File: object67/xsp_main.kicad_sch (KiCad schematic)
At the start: 67 parts, among them IC5 TPS7A4701RGWT, IC6 TPS7A3301RGWR, J2 PJ-037A, J3 Power In, J4 216700-0249, U10 ADP5070AREZ, U11 TPS62912, U7 TPS7A2050PDQNR, U8 TPS7A2033PDQNR, U9 TPS7A2033PDQNR

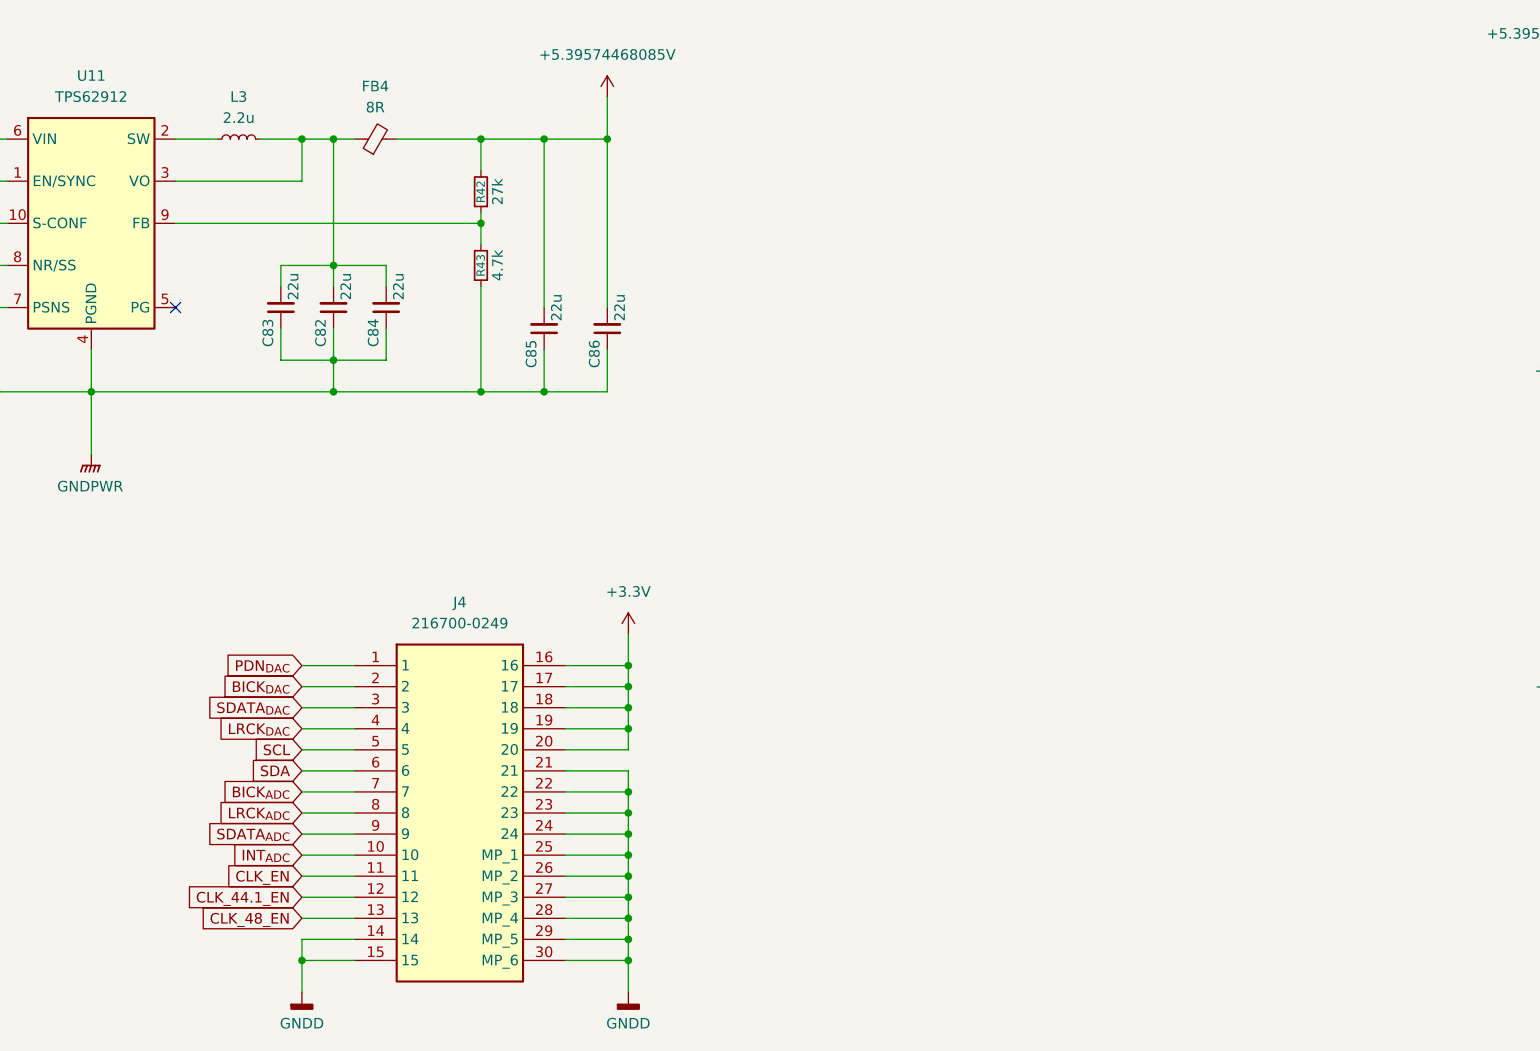
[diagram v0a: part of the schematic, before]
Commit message: Start layout
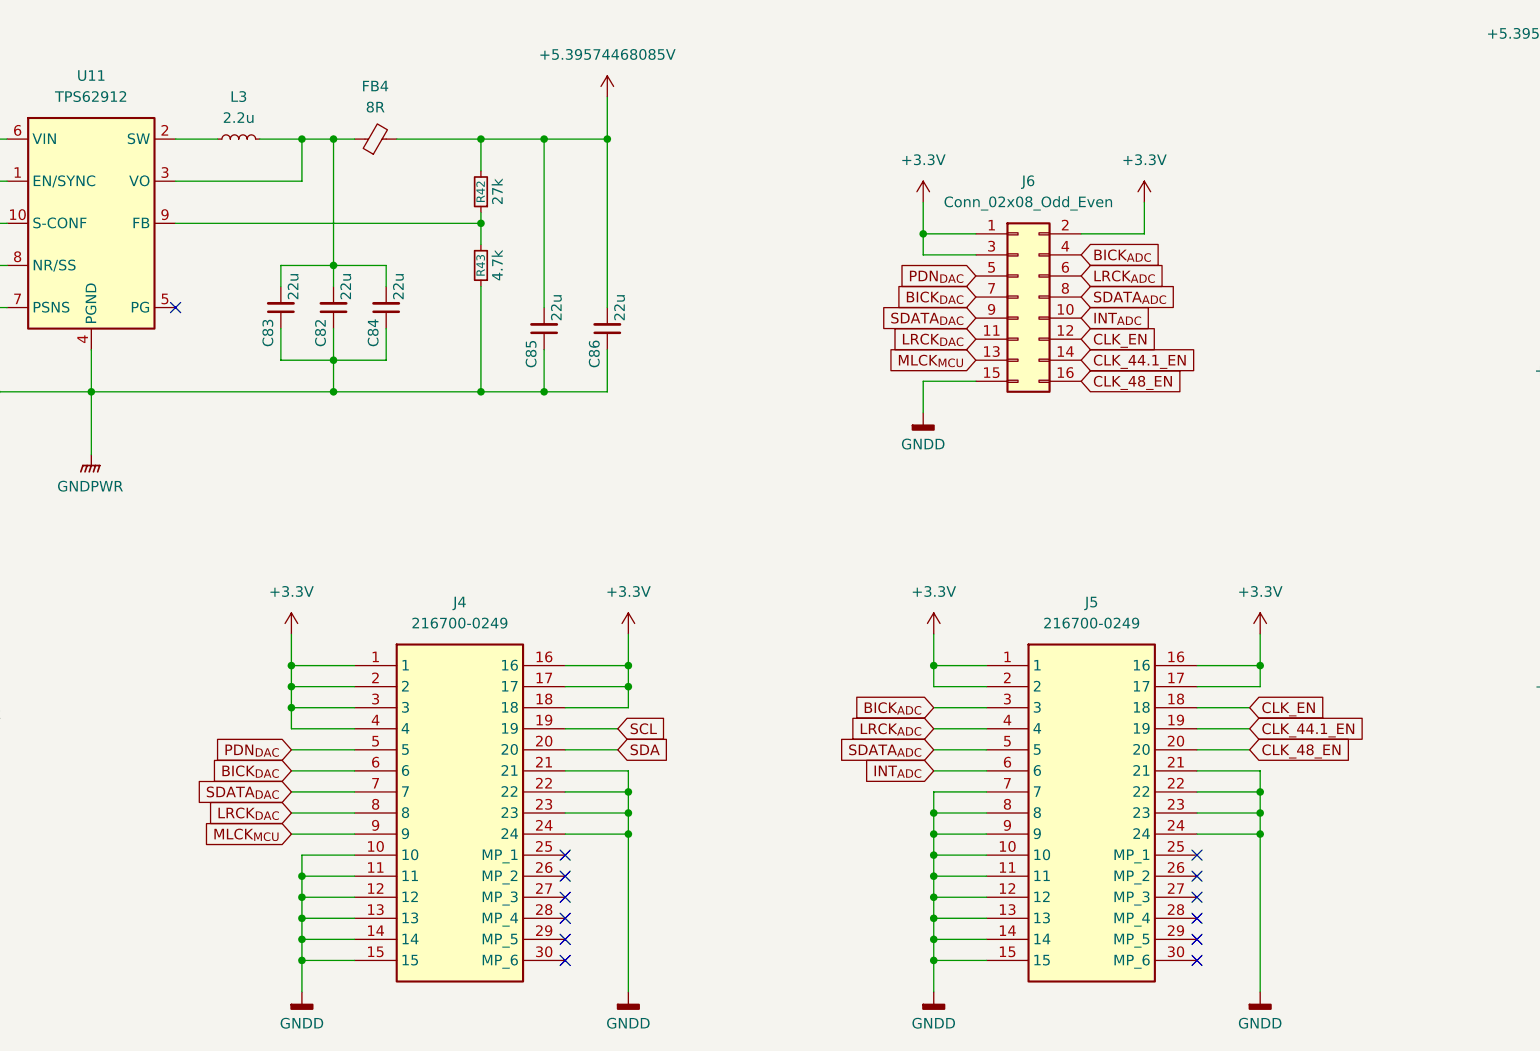
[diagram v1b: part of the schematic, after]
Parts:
- added J5: 216700-0249, object67:2167000249, symbol object67:216700-0249
- added J6: Conn_02x08_Odd_Even, Connector_PinHeader_2.54mm:PinHeader_2x08_P2.54mm_Horizontal, symbol Connector_Generic:Conn_02x08_Odd_Even
- J3: footprint Connector_PinHeader_2.54mm:PinHeader_1x01_P2.54mm_Vertical -> TestPoint:TestPoint_2Pads_Pitch5.08mm_Drill1.3mm
- R35, R36, R37, R38, R39, R40, R42, R43, R44, R45: footprint (none) -> Resistor_SMD:R_0805_2012Metric
- R41: footprint (none) -> Resistor_SMD:R_0603_1608Metric
- TP1, TP2, TP3, TP4: footprint (none) -> TestPoint:TestPoint_Pad_D2.0mm
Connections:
- net +3.3V: now also J4.1, J4.2, J4.3, J4.4, J5.1, J5.16, J5.17, J5.2, J6.1 (Pin_1), J6.2 (Pin_2), J6.3 (Pin_3); no longer J4.19, J4.20
- net BICK_{ADC}: now also J5.3, J6.4 (Pin_4); no longer J4.7
- net BICK_{DAC}: now also J4.6, J6.7 (Pin_7); no longer J4.2
- net CLK_44.1_EN: now also J5.19, J6.14 (Pin_14); no longer J4.12
- net CLK_48_EN: now also J5.20, J6.16 (Pin_16); no longer J4.13
- net CLK_EN: now also J5.18, J6.12 (Pin_12); no longer J4.11
- net GNDD: now also J4.10, J4.11, J4.12, J4.13, J5.10, J5.11, J5.12, J5.13, J5.14, J5.15, J5.21, J5.22, J5.23, J5.24, J5.7, J5.8, J5.9, J6.15 (Pin_15); no longer J4.25 (MP_1), J4.26 (MP_2), J4.27 (MP_3), J4.28 (MP_4), J4.29 (MP_5), J4.30 (MP_6)
- net INT_{ADC}: now also J5.6, J6.10 (Pin_10); no longer J4.10
- net LRCK_{ADC}: now also J5.4, J6.6 (Pin_6); no longer J4.8
- net LRCK_{DAC}: now also J4.8, J6.11 (Pin_11); no longer J4.4
- net PDN_{DAC}: now also J4.5, J6.5 (Pin_5); no longer J4.1
- net SCL: now also J4.19; no longer J4.5
- net SDA: now also J4.20; no longer J4.6
- net SDATA_{ADC}: now also J5.5, J6.8 (Pin_8); no longer J4.9
- net SDATA_{DAC}: now also J4.7, J6.9 (Pin_9); no longer J4.3
- new net MLCK_{MCU}: J4.9, J6.13 (Pin_13)
- no-connect marks 22 -> 34
